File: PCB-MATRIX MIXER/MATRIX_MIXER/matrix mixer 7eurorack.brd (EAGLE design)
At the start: 150.8 x 119.1 mm, 161 parts, among them IC4 TL072D, IC5 TL072D, IC6 TL072D, IC7 TL072D, IC8 TL072D, IC9 TL072D, J16 M05X2PTH, Q1 MMBT3904, Q2 MMBT3904, Q3 MMBT3904, Q4 MMBT3904, Q5 MMBT3904, Q6 MMBT3904

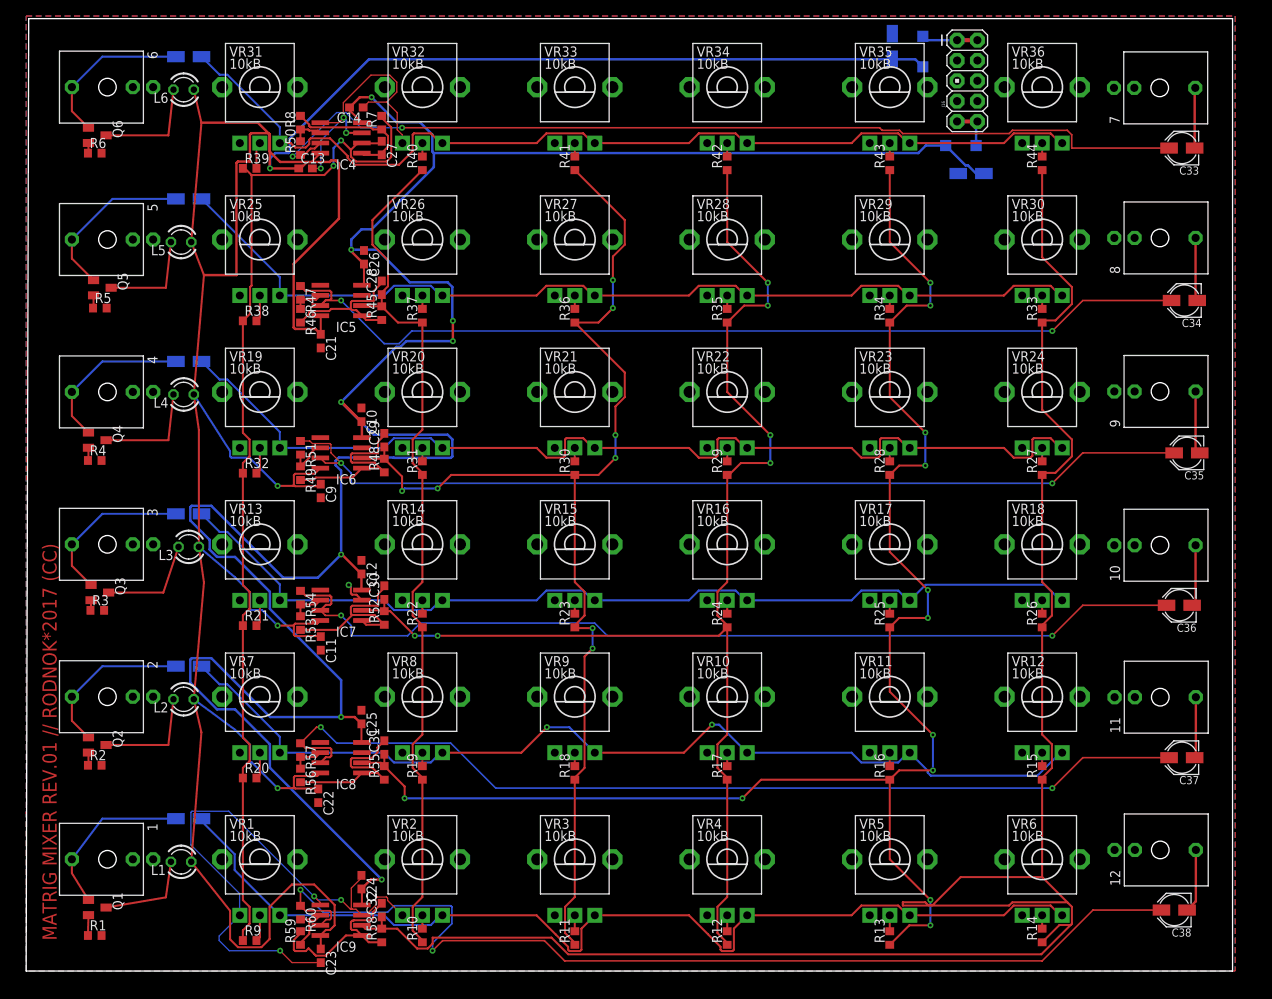
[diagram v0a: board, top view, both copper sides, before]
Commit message: Add files via upload
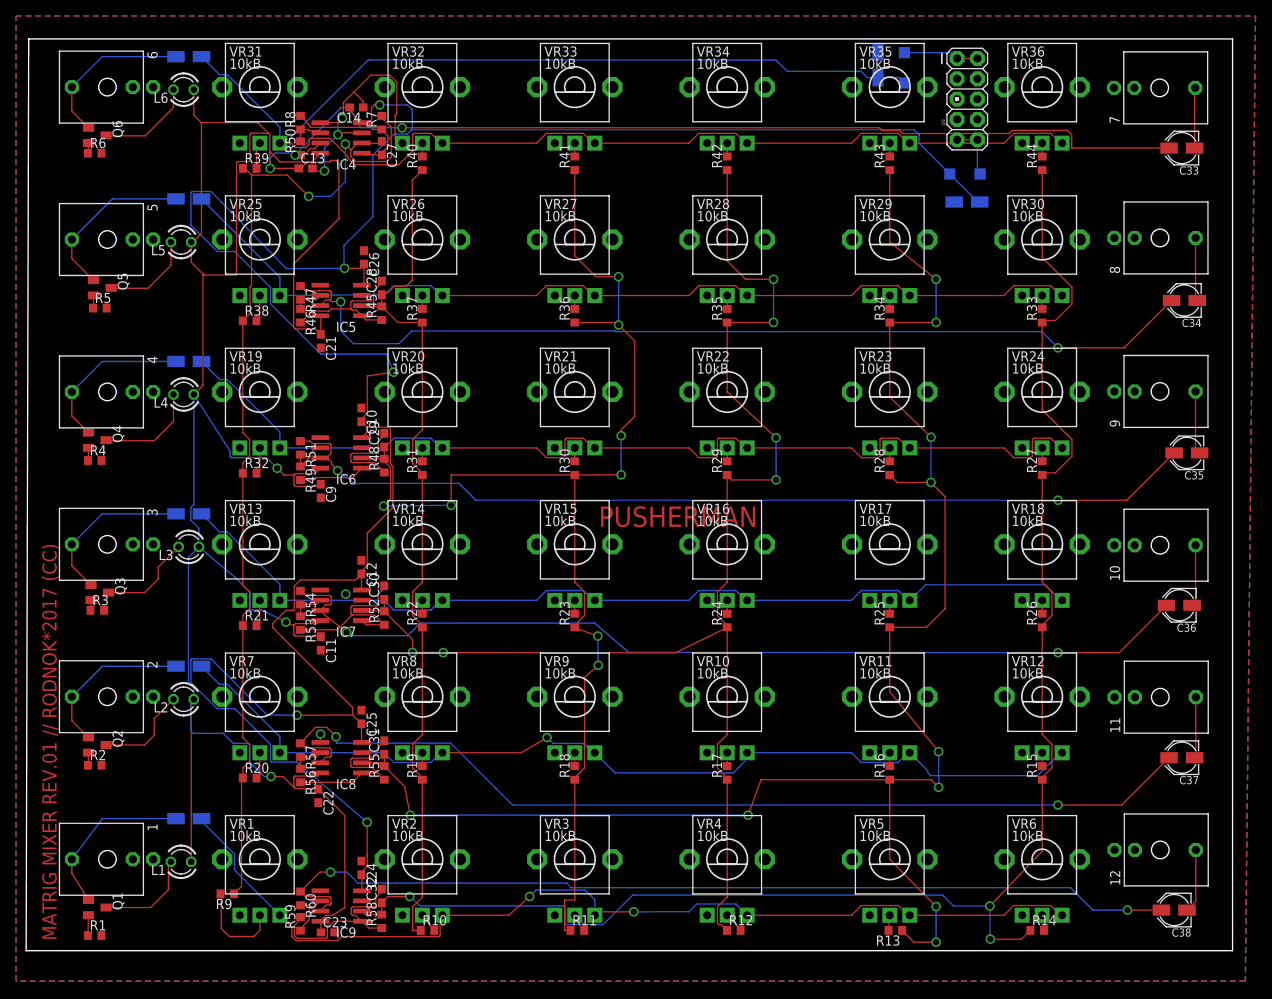
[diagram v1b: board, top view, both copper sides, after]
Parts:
- moved R9 6.48 mm to (27.7, 5.84), turned to 180 degrees
- moved C2 3.59 mm to (120.1, 92.3)
- moved D2 3.59 mm to (119.9, 95.8)
- moved D1 3.06 mm to (112.3, 109.1)
- moved C23 3.05 mm to (40.3, 1.02), turned to 0 degrees
- moved C1 2.90 mm to (109.0, 109.5)
- moved J16 2.29 mm to (120.2, 105.2)
- moved C24 1.78 mm to (44.5, 9.08)
- moved C32 1.78 mm to (47.0, 5.59)
- moved R59 1.78 mm to (36.8, 2.10)
- moved R60 1.78 mm to (36.8, 5.27)
- moved R58 1.78 mm to (47.0, 2.41)
- moved IC9 1.78 mm to (41.9, 4.32)
- moved R12 1.26 mm to (91.0, 1.27), turned to 0 degrees
- moved R13 1.18 mm to (111.2, 1.27), turned to 180 degrees
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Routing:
- net GND: track 115.3 -> 37.5 mm, vias 7 -> 5
- net N$67: track 245.3 -> 199.4 mm, vias 0 -> 3
- net VEE: track 338.8 -> 315.8 mm, vias 8 -> 5
- net VCC: track 389.8 -> 374.5 mm
- net N$96: track 131.0 -> 117.2 mm
- net N$66: track 198.3 -> 210.6 mm, vias 12 -> 10
- net N$64: track 147.4 -> 156.8 mm
- net N$1: track 3.33 -> 11.8 mm
- net N$65: track 161.6 -> 169.1 mm
- net N$62: track 133.2 -> 130.6 mm
- net INPUT_1: track 127.9 -> 125.4 mm, vias 0 -> 2
- net N$80: track 117.9 -> 120.3 mm
- net N$44: track 7.03 -> 9.42 mm
- net N$92: track 120.9 -> 123.0 mm
- net INPUT_2: track 123.3 -> 121.6 mm, vias 2 -> 1
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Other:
- board size 150.8 x 119.1 mm -> 150.8 x 114 mm
- board text added: "PUSHERMAN"
